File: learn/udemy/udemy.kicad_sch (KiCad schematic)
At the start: 13 parts, among them J1 Screw_Terminal_01x02, J2 Screw_Terminal_01x02, J3 Screw_Terminal_01x02, U1 L7809, U2 L7805

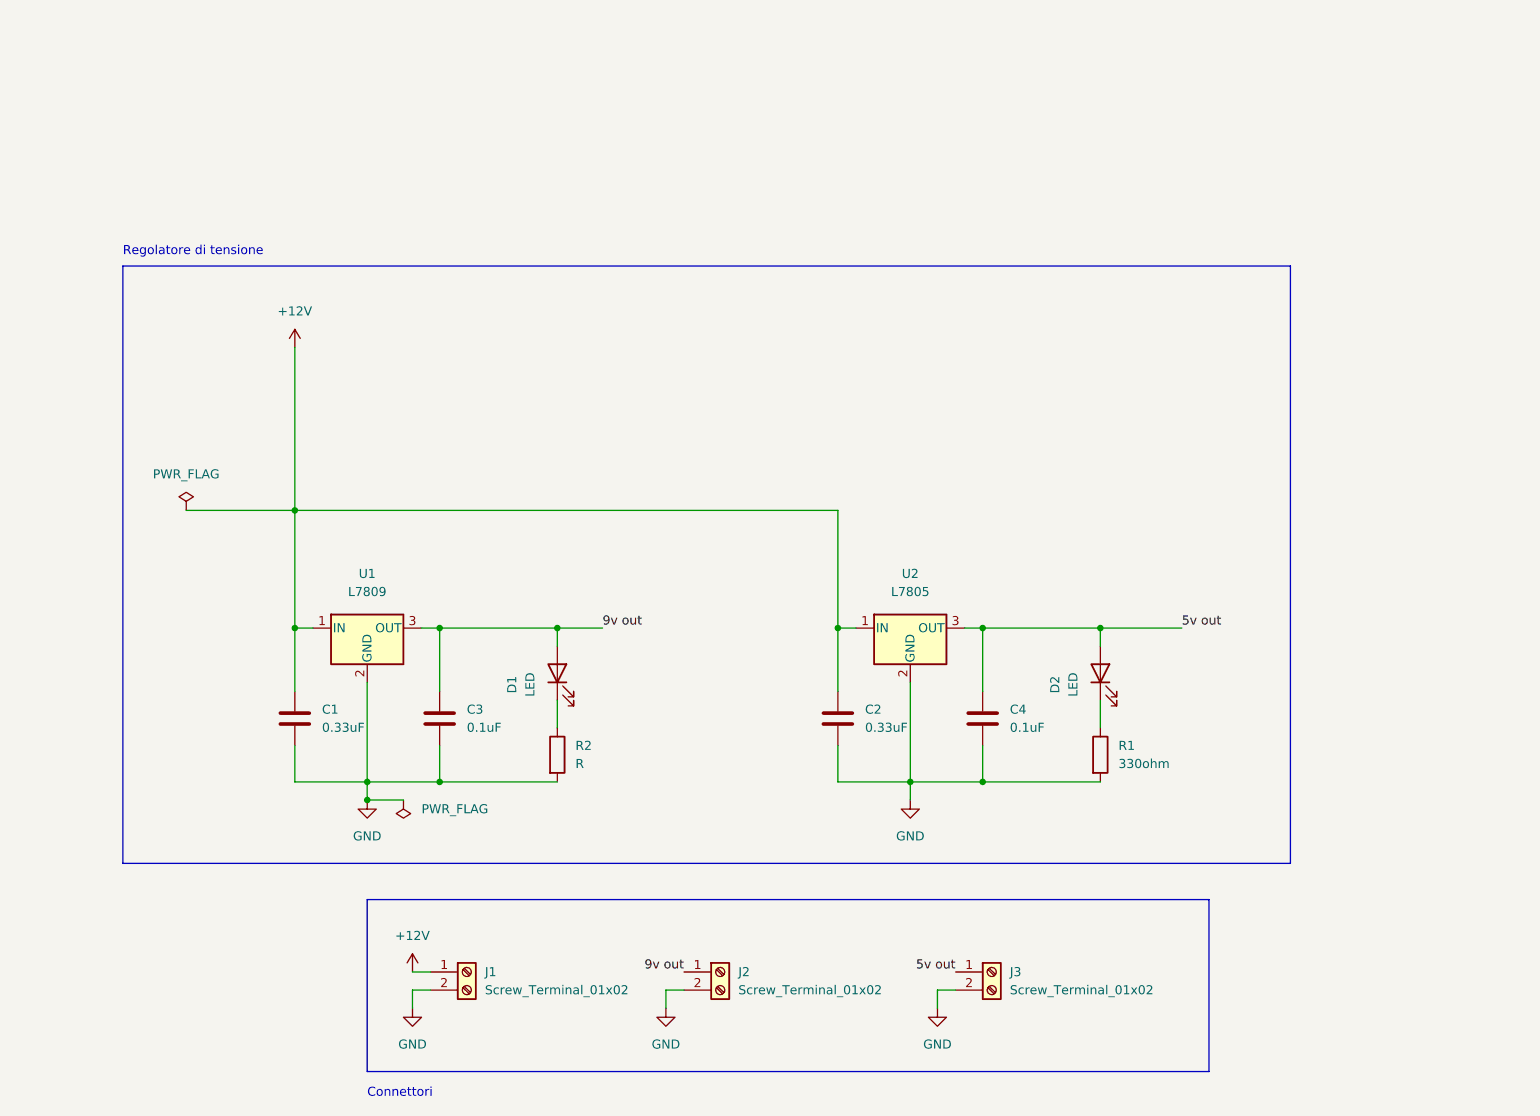
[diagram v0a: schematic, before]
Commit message: 05/01/23 modifiche al circuito elettrico
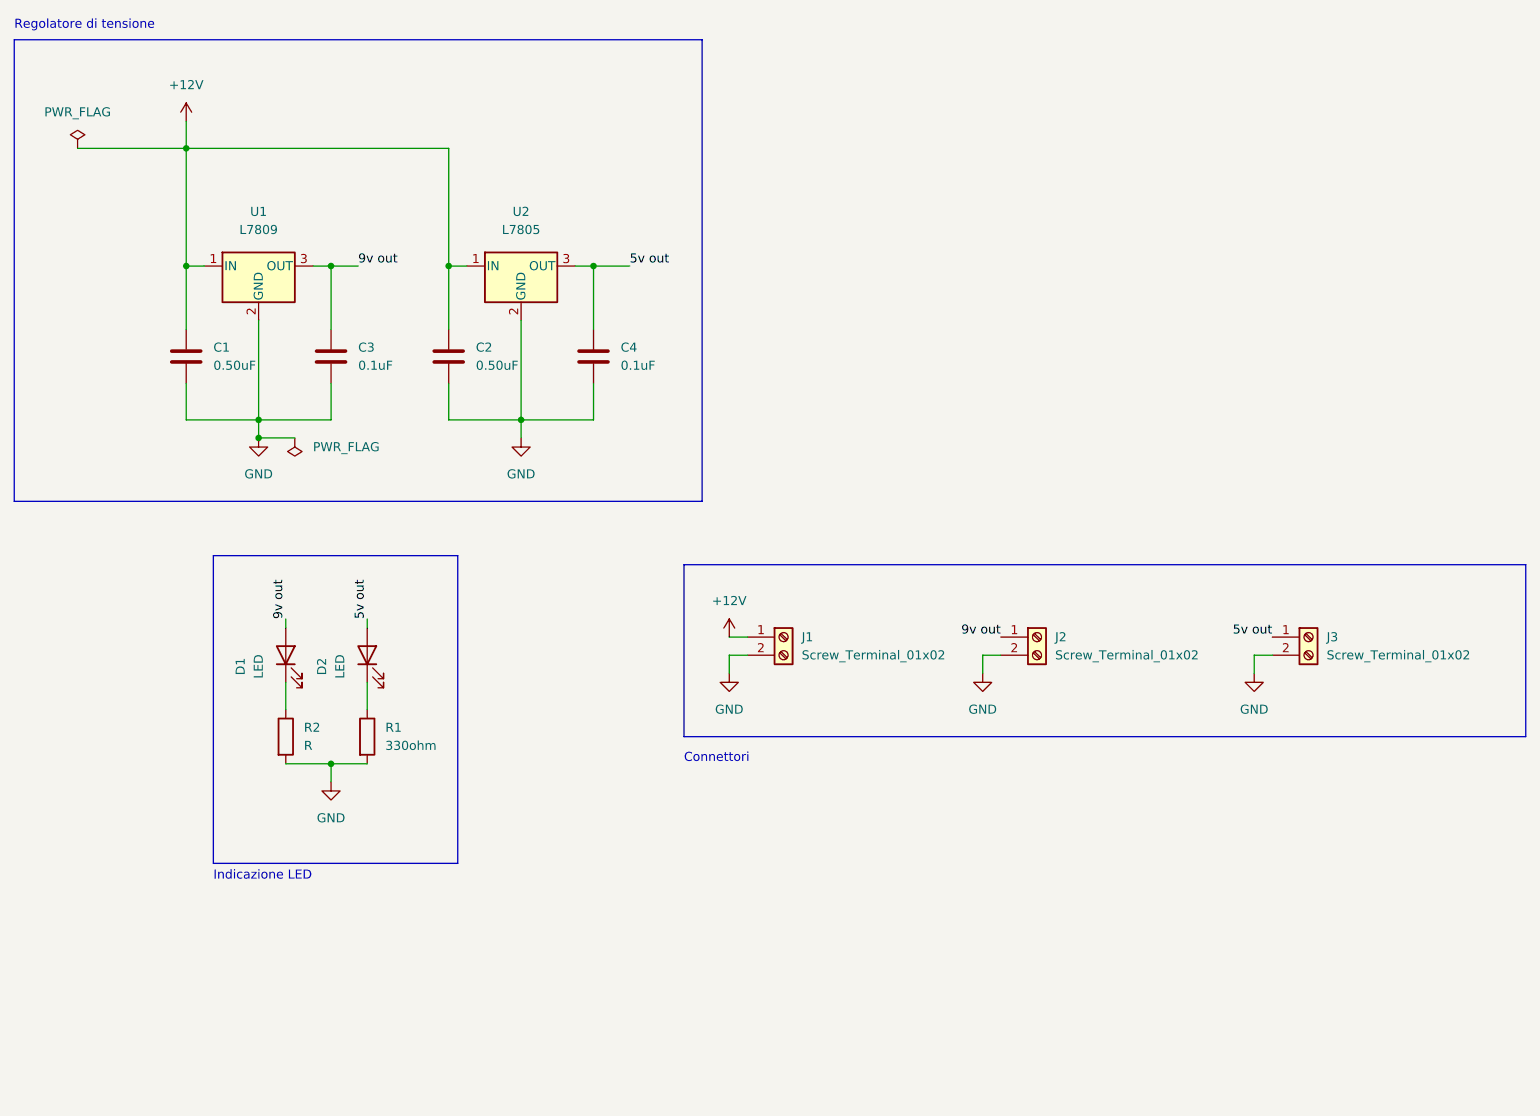
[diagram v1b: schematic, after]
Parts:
- C1, C2: value 0.33uF -> 0.50uF
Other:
- note added: "Indicazione LED"
- moved on the sheet: C1, C2, C3, C4, D1, D2, J1, J2, J3, R1, R2, U1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
